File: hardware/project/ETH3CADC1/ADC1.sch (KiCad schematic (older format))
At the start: 53 parts, among them U201 DG211, U202 DG211B, U203 OPA2192, U204 DG419DY, U205 OPA140, U206 LT5400-100k-100k, U207 LT5400-5k-1k, U208 OPA177, U209 OPA140, U210 LT5400-10k-10k, U211 OPA192, U212 LM311

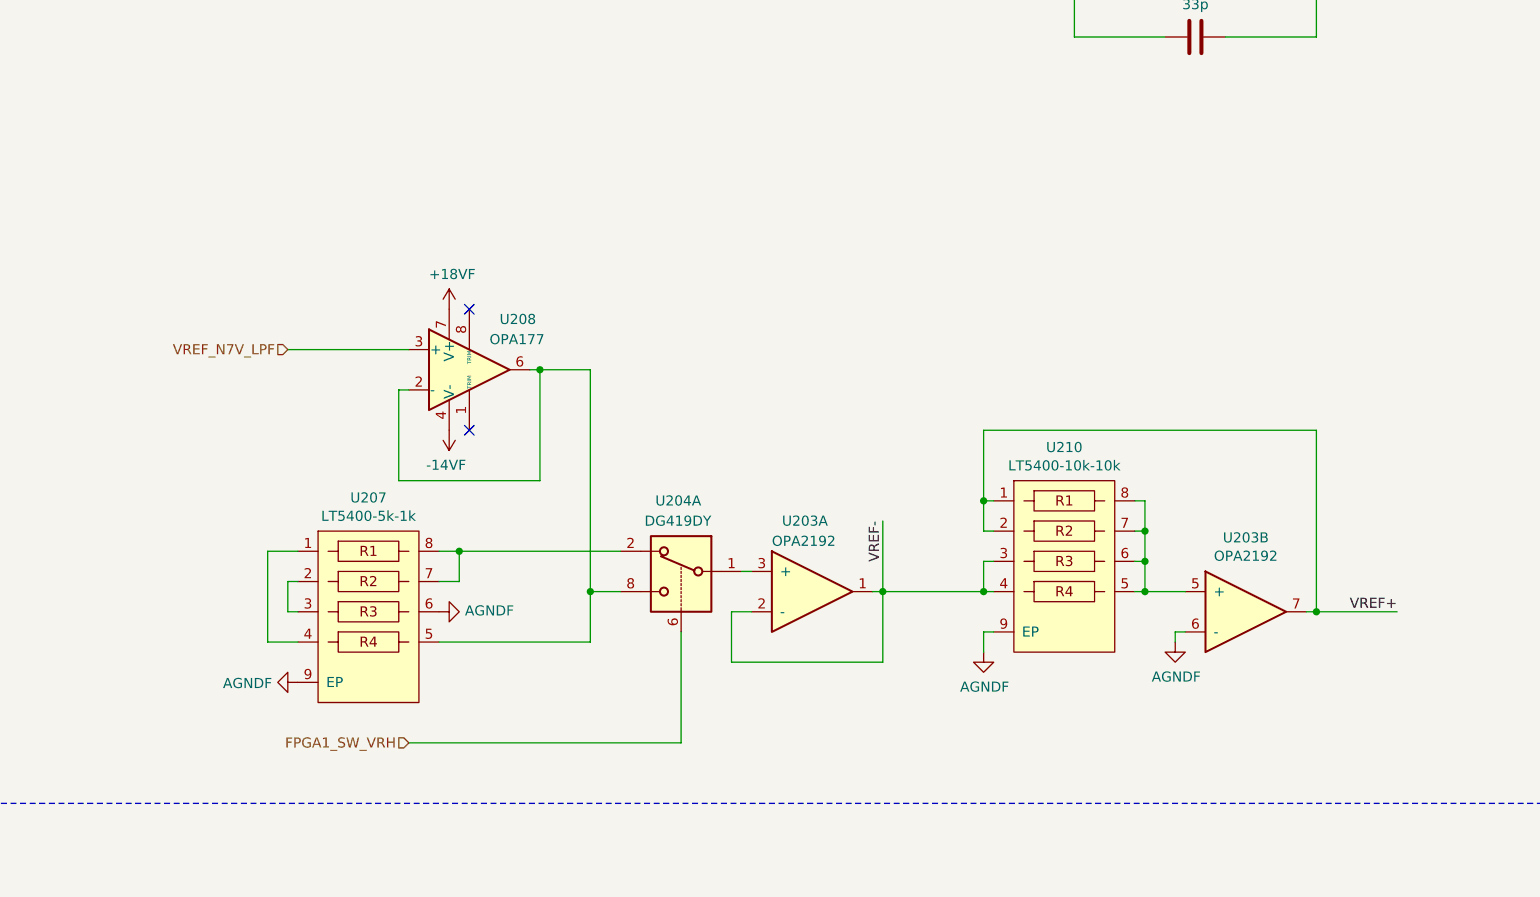
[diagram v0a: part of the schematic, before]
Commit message: PCB layout
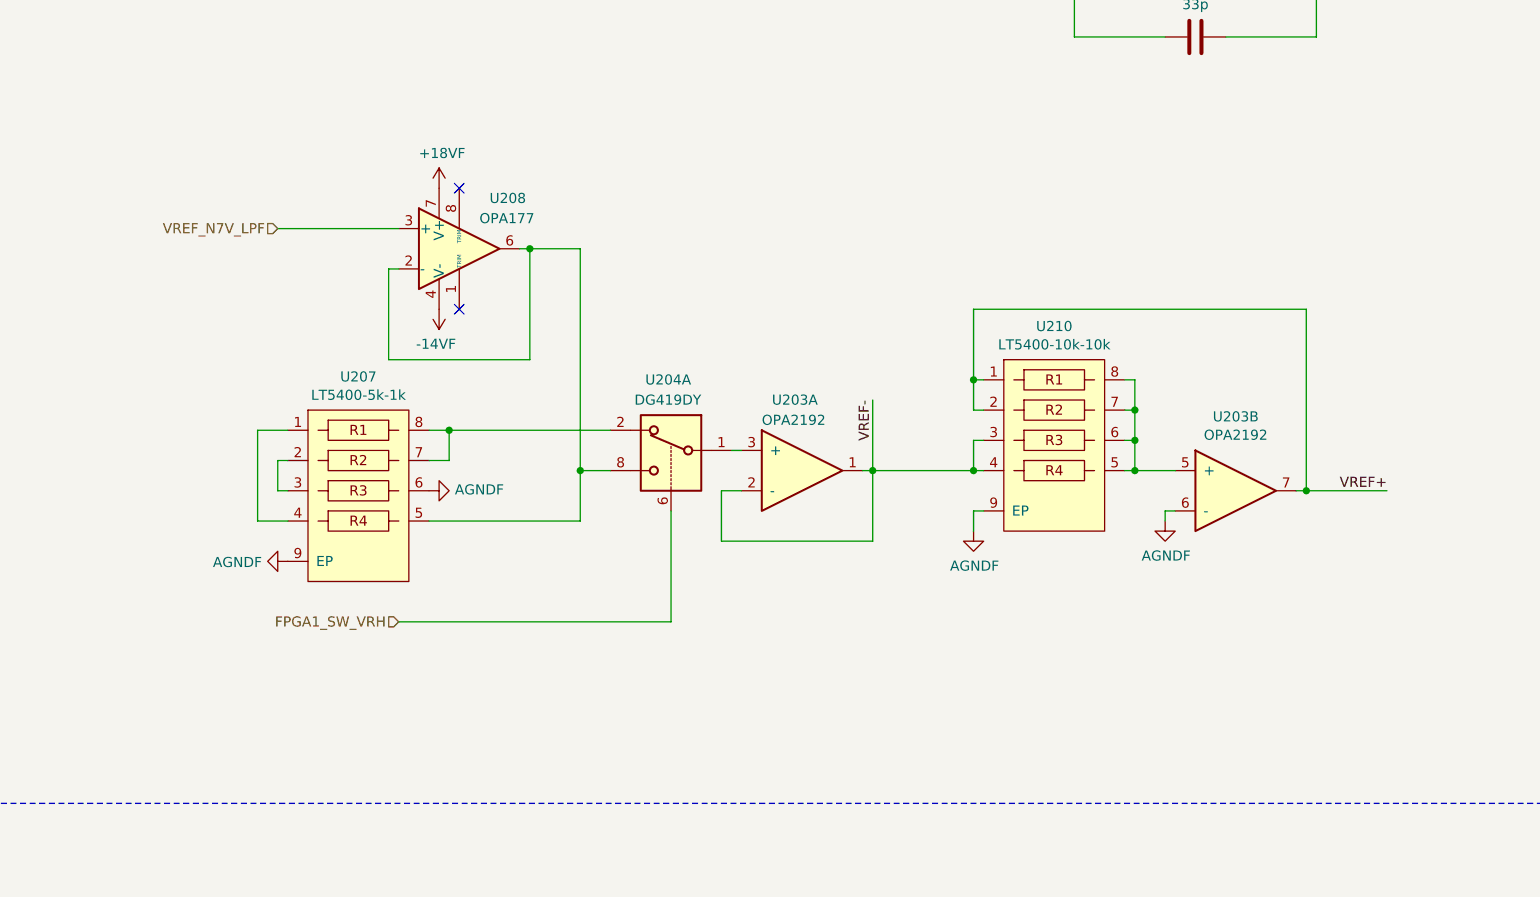
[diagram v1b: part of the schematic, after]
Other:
- moved on the sheet: U203A, U203B, U204A, U207, U208, U210
